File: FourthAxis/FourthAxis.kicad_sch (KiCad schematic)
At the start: 31 parts, among them J1 36V, J2 DRIVER_CONN, J3 ENC_CONN, J4 HW_CONN, J5 SCREEN_CONN, J6 PROG_HEADER, SW29 BOOT, SW30 RESET, U1 ESP32-WROOM-32

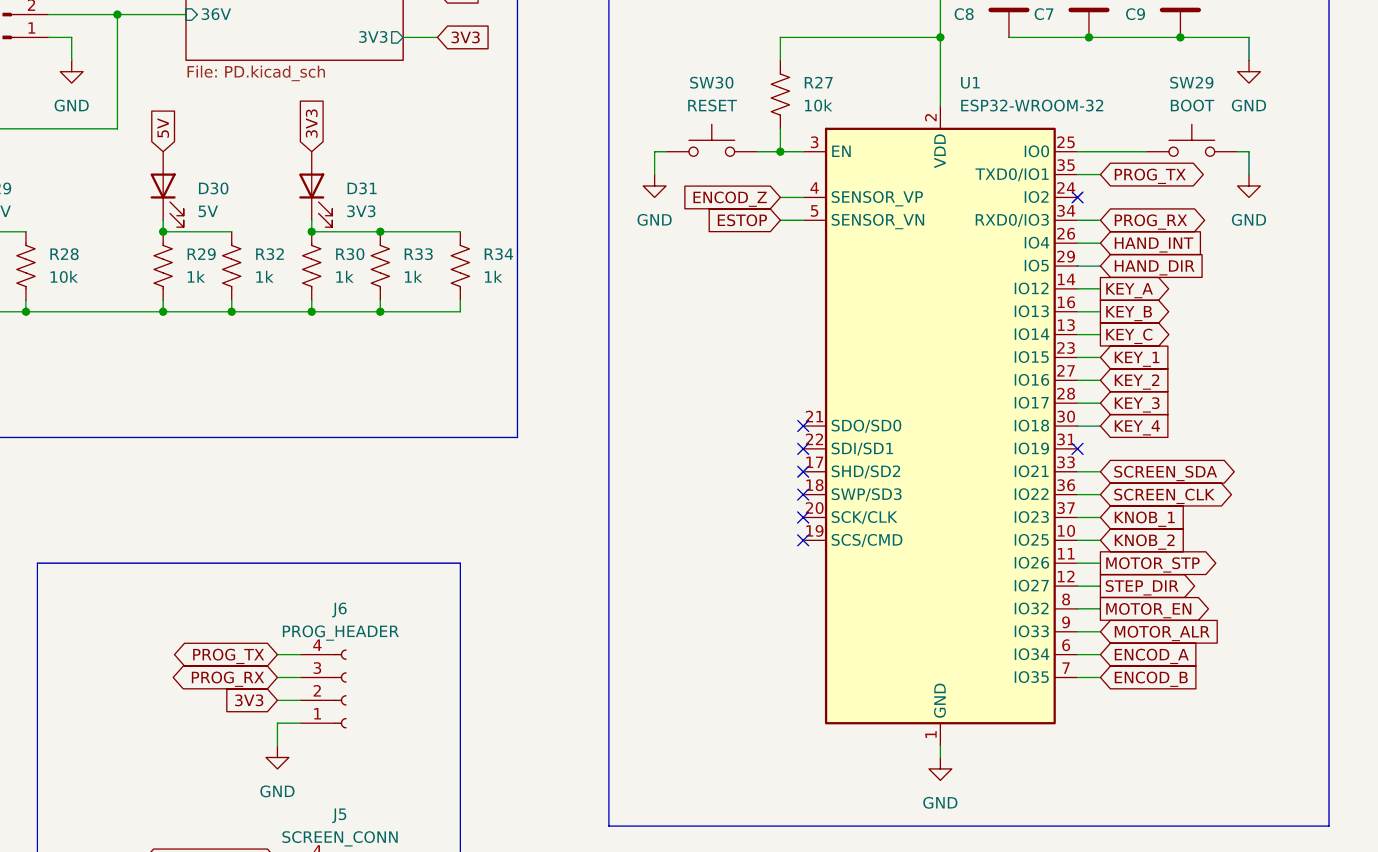
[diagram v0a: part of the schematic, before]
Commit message: started routing
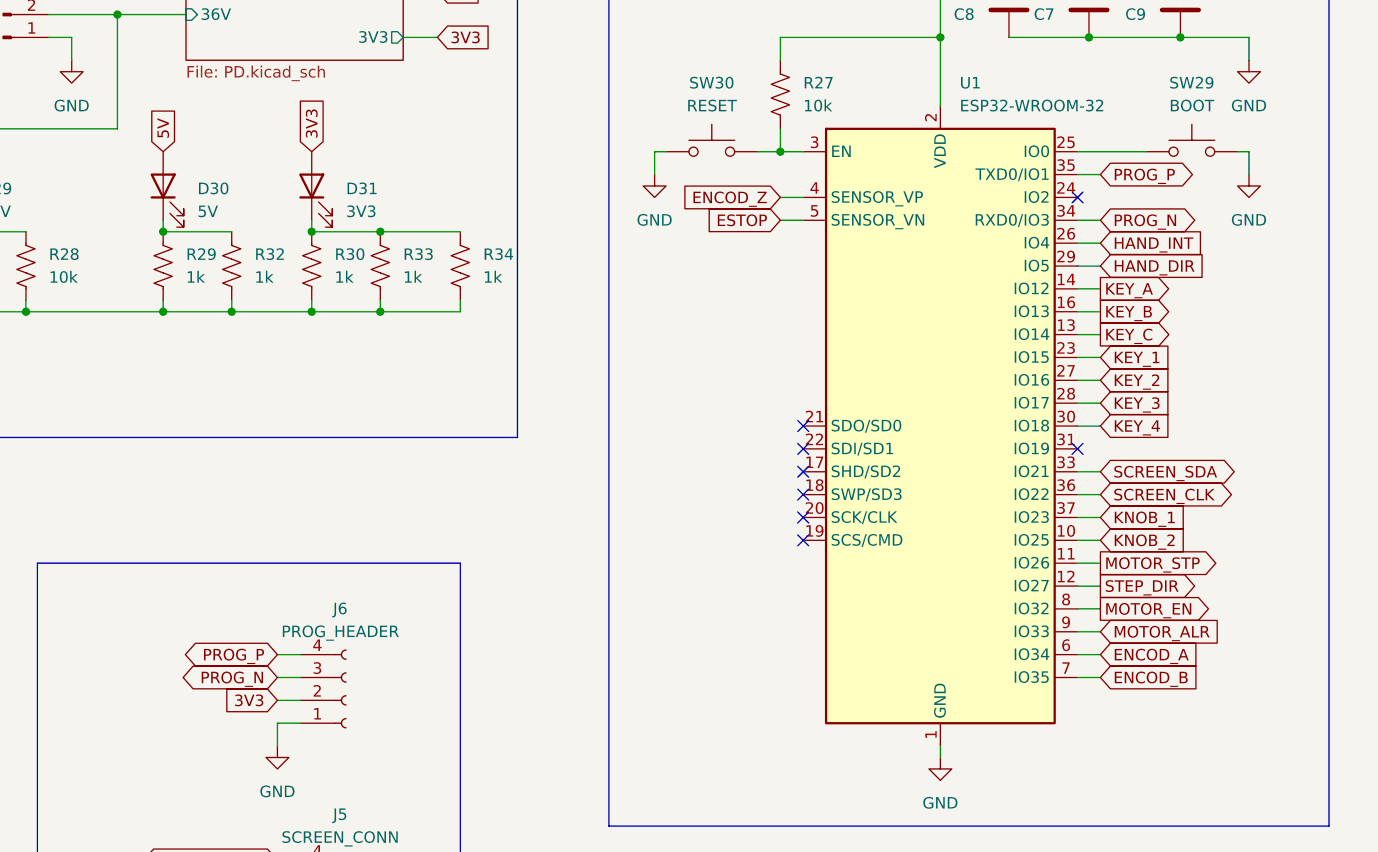
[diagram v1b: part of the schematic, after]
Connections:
- net PROG_RX renamed PROG_N
- net PROG_TX renamed PROG_P
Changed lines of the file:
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@@
 		)
 	)
-	(global_label "PROG_RX"
+	(global_label "PROG_N"
 		(shape bidirectional)
 		(at 151.13 66.04 0)
@@
 		)
 		(property "Intersheetrefs" "${INTERSHEET_REFS}"
-			(at 163.0011 66.04 0)
+			(at 161.8521 66.04 0)
 			(hide yes)
 			(show_name no)
@@
 		)
 	)
-	(global_label "PROG_RX"
+	(global_label "PROG_N"
 		(shape bidirectional)
 		(at 59.69 116.84 180)
@@
 		)
 		(property "Intersheetrefs" "${INTERSHEET_REFS}"
-			(at 47.8189 116.84 0)
+			(at 48.9679 116.84 0)
 			(hide yes)
 			(show_name no)
@@
 		)
 	)
-	(global_label "PROG_TX"
+	(global_label "PROG_P"
 		(shape bidirectional)
 		(at 151.13 60.96 0)
@@
 		)
 		(property "Intersheetrefs" "${INTERSHEET_REFS}"
-			(at 162.6987 60.96 0)
+			(at 161.7916 60.96 0)
 			(hide yes)
 			(show_name no)
@@
 		)
 	)
-	(global_label "PROG_TX"
+	(global_label "PROG_P"
 		(shape bidirectional)
 		(at 59.69 114.3 180)
@@
 		)
 		(property "Intersheetrefs" "${INTERSHEET_REFS}"
-			(at 48.1213 114.3 0)
-			(hide yes)
-			(show_name no)
+			(at 49.0284 114.3 0)
+			(hide yes)
+			(show_name no)
